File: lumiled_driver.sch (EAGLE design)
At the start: 39 parts, among them Q1 IRF520, Q10 2N3904, Q11 2N3904, Q12 2N3904, Q2 2N3904, Q3 IRF520, Q4 2N3904, Q5 IRF520, Q6 2N3904, Q7 IRF520, Q8 IRF520, Q9 IRF520

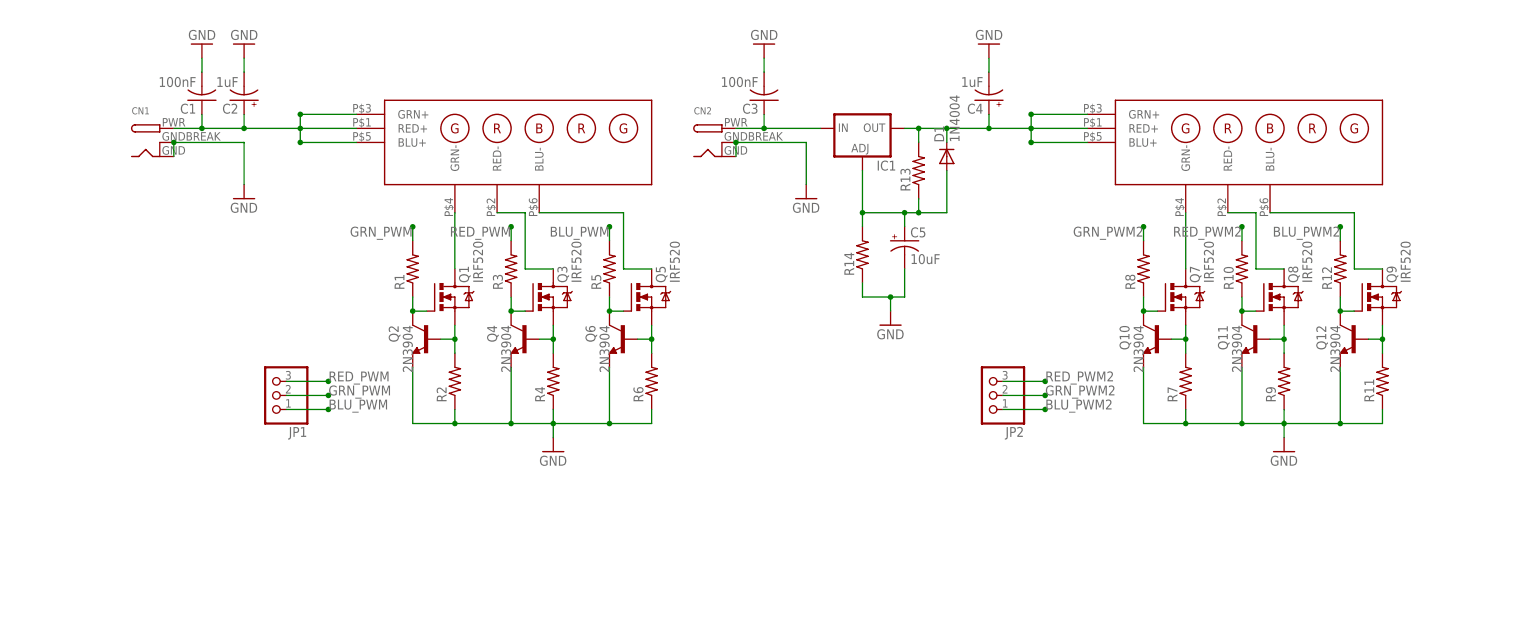
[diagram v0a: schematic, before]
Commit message: frankly, I've forgotten all the changes I've made but it's a lot
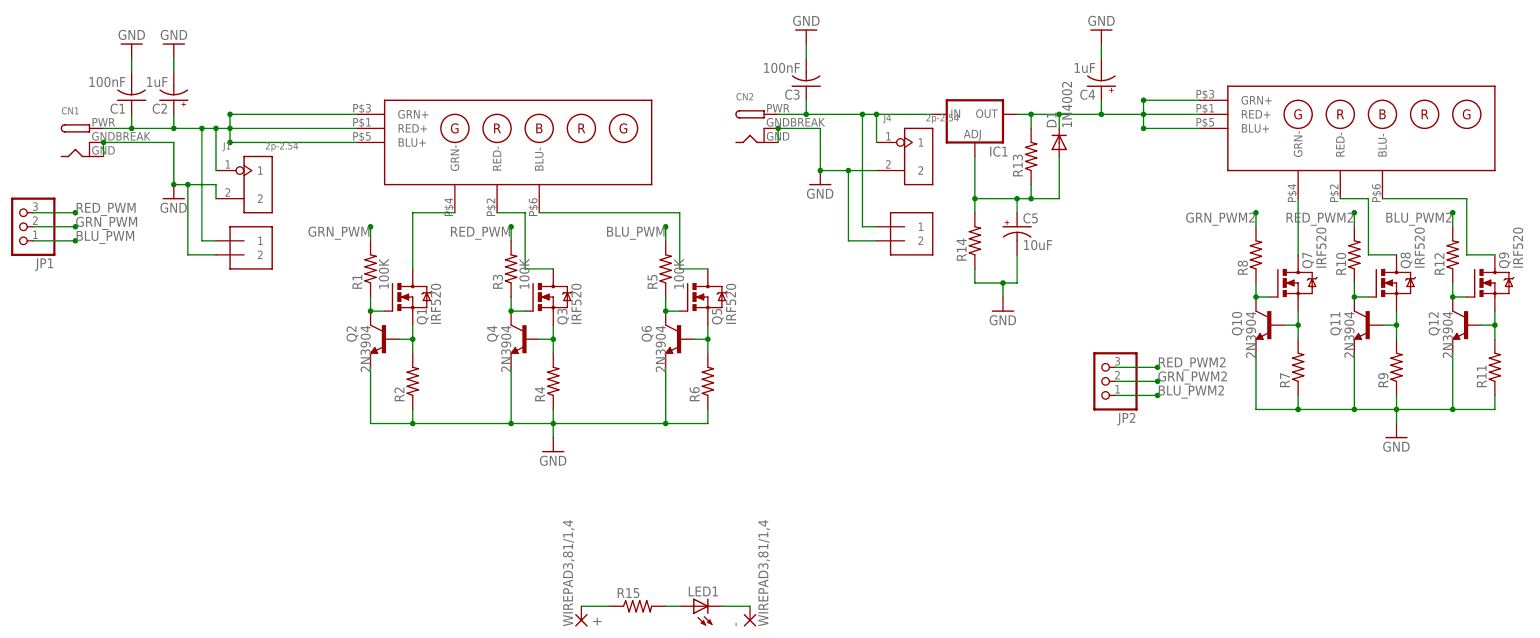
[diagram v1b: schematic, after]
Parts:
- added +, -: WIREPAD3,81/1,4, wirepad:WIREPAD3,81/1,4
- added J1, J4: 2p-2.54, Seeed-Connector:DIP-BLACK-MALE-HEADER-VERT(2P-2.54)
- added J2, J3: 1X2-3.5MM, adafruit:1X2-3.5MM
- added LED1: (no value), led:LED3MM
- added R15: (no value), resistor:R-US_0207/12
- D1: value 1N4004 -> 1N4002
- R1, R3, R5: value (none) -> 100K
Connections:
- new net N$41: LED1.A, R15.2
- new net N$42: +.P, R15.1
- new net N$43: -.P, LED1.C
- net +VIN: now also J1.1, J2.1
- net GND: now also J1.2, J2.2, J3.2, J4.2
- net N$11: now also J3.1, J4.1
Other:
- moved on the sheet: C1, C2, C3, C4, C5, CN1, CN2, D1, IC1, JP1, JP2, Q1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
